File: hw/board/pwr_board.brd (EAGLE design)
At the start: 101.6 x 76.2 mm, 41 parts, among them IC1 7805T

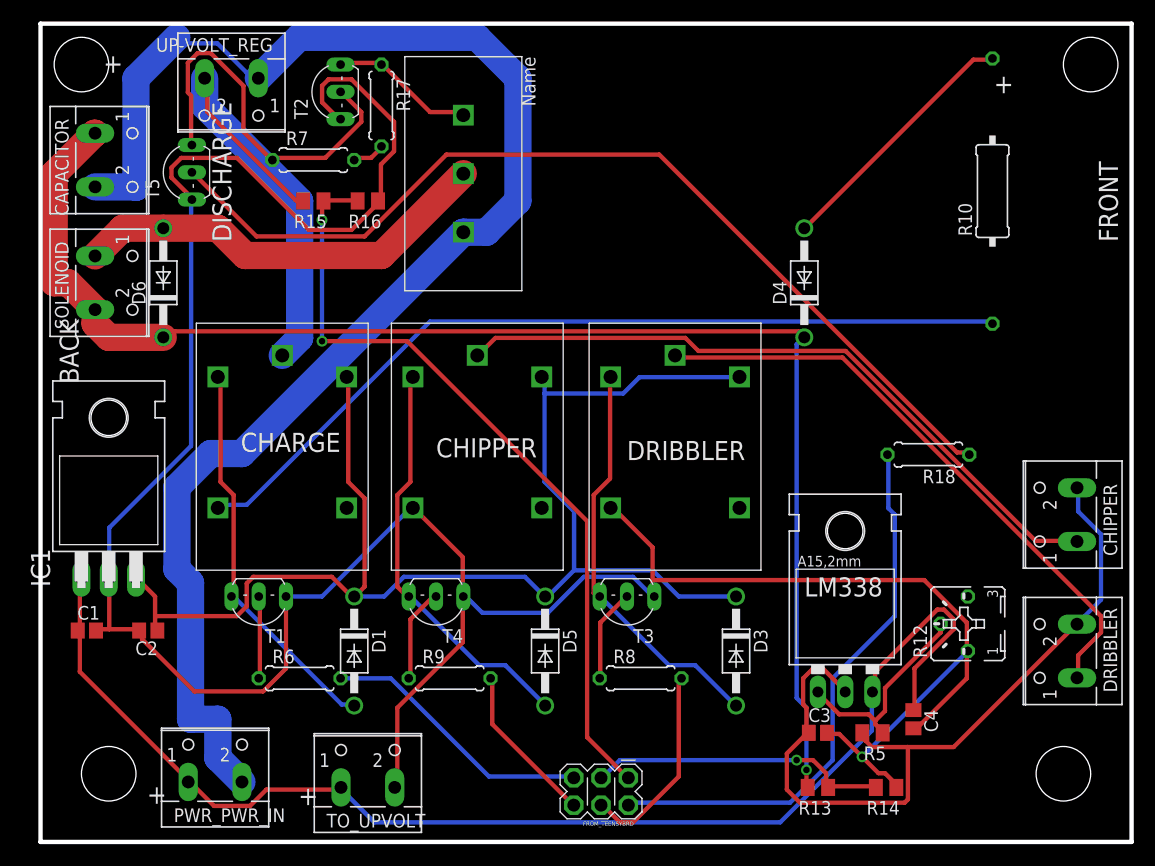
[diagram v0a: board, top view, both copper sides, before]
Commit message: Pwr board routing
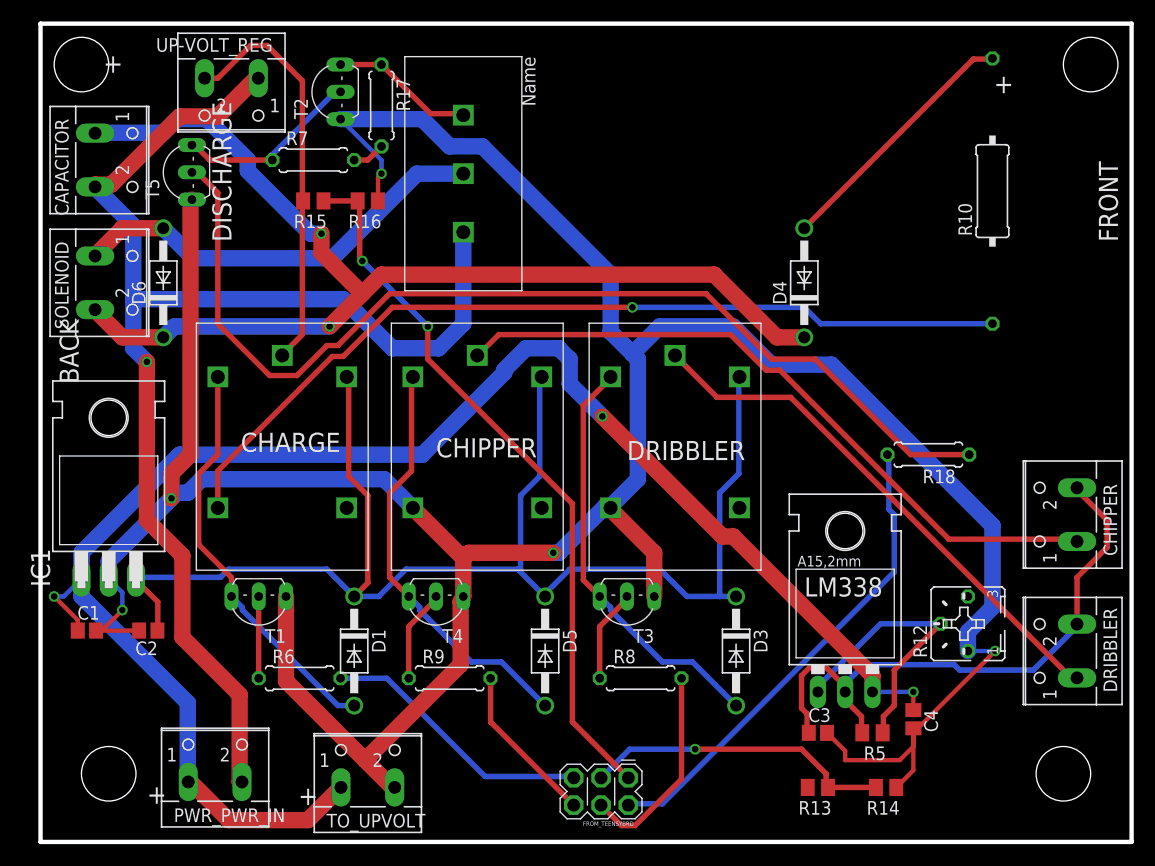
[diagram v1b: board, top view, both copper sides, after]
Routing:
- net GND: track 261.8 -> 300.8 mm, vias 1 -> 5
- net VCC: track 119.3 -> 152.4 mm, vias 0 -> 3
- net N$13: track 131.3 -> 105.8 mm, vias 1 -> 2
- net N$4: track 36.1 -> 17.5 mm
- net GND_PWR: track 141.3 -> 122.8 mm, vias 0 -> 1
- net +12V: track 73.7 -> 56.1 mm
- net N$14: track 45.8 -> 38.1 mm
- net N$2: track 19.4 -> 26.8 mm
- net N$3: track 89.6 -> 96.7 mm
- net PWR_DISCHARGE: track 51.9 -> 45.0 mm
- net N$22: track 56.5 -> 50.0 mm
- net PWR_READ_250: track 73.4 -> 67.5 mm
- net N$10: track 79.4 -> 82.5 mm, vias 0 -> 1
- net +5V: track 126.7 -> 129.3 mm
- net N$6: track 37.0 -> 38.2 mm
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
